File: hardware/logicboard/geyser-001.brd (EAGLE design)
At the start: 47 x 47 mm, 13 parts, among them T1 2SC1815

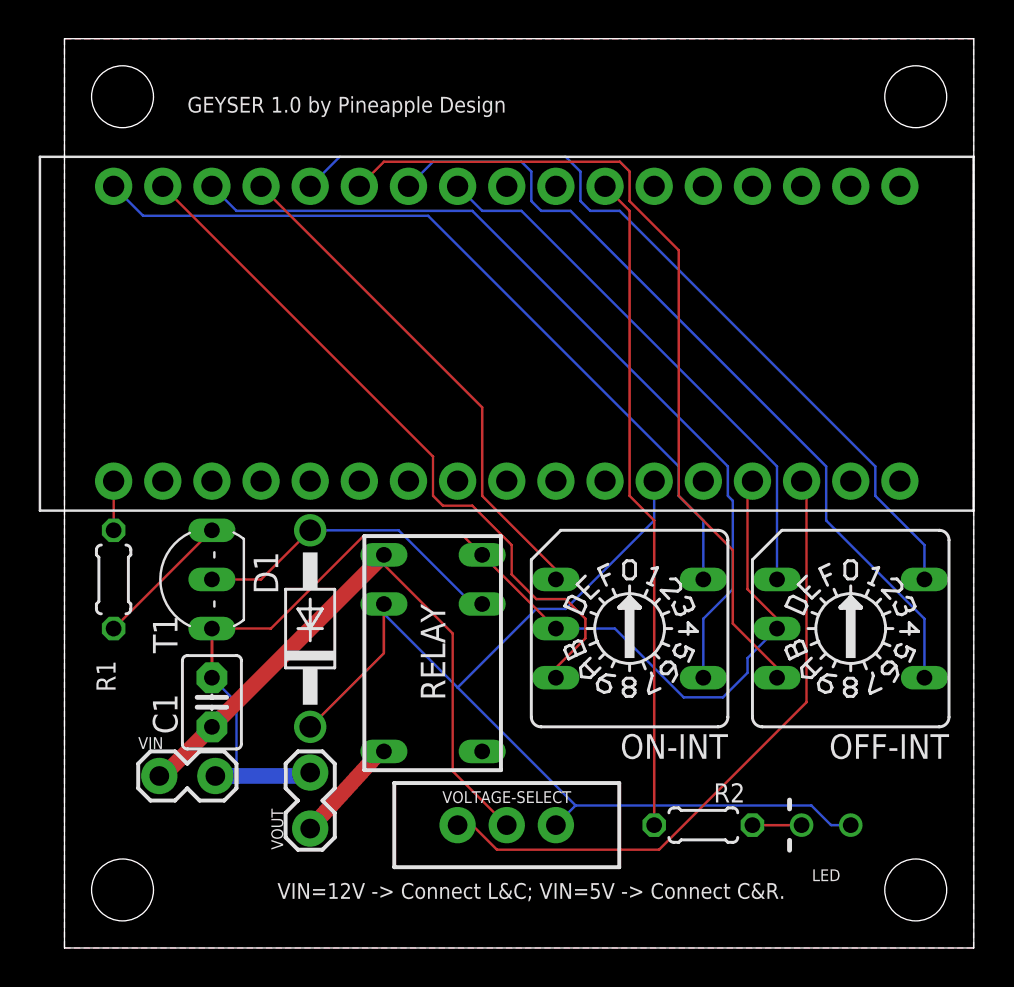
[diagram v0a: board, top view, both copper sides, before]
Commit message: Changed layout rule.
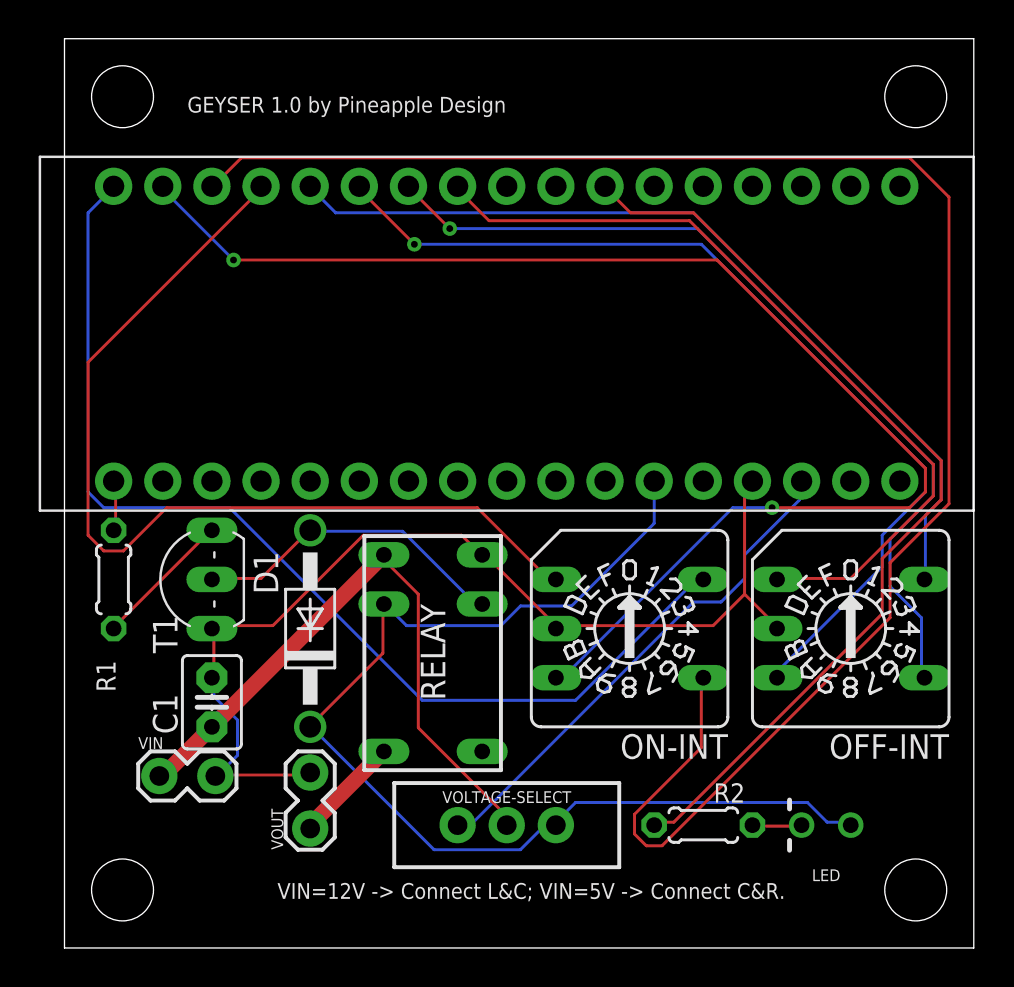
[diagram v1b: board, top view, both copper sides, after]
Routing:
- net N$9: track 44.3 -> 90.4 mm
- net N$8: track 36.9 -> 69.9 mm, vias 0 -> 2
- net N$10: track 26.6 -> 48.7 mm
- net LEDDRIVE: track 34.1 -> 48.8 mm
- net N$11: track 28.3 -> 42.1 mm
- net N$7: track 41.6 -> 55.2 mm
- net VIN: track 33.3 -> 26.4 mm
- net N$5: track 44.0 -> 49.4 mm, vias 0 -> 1
- net VCC: track 54.5 -> 59.0 mm
- net GND: track 58.3 -> 54.5 mm
- net N$6: track 42.6 -> 45.8 mm, vias 0 -> 1
- net N$2: track 44.3 -> 45.0 mm
- removed copper zone on layer 1, net GND
- removed copper zone on layer 16, net GND
